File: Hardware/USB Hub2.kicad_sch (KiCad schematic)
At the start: 67 parts, among them J1 Conn_01x07_Male, J10 Conn_01x04_Male, J11 USB_C_Receptacle, J12 USB_C_Receptacle, J2 Conn_01x04_Male, J3 Conn_01x02_Male, J4 Conn_01x02_Male, J5 Conn_01x02_Male, J6 Conn_01x02_Male, J7 Conn_01x08_Male, J8 QWIIC_Vertical, J9 QWIIC_Stack_II, U1 TUSB2036, U2 AP2112K-3.3, U3 TPS2550DBVTG4, U4 TPS2550DBVTG4, U5 TPS2550DBVTG4, X1 ASE-48.000MHz

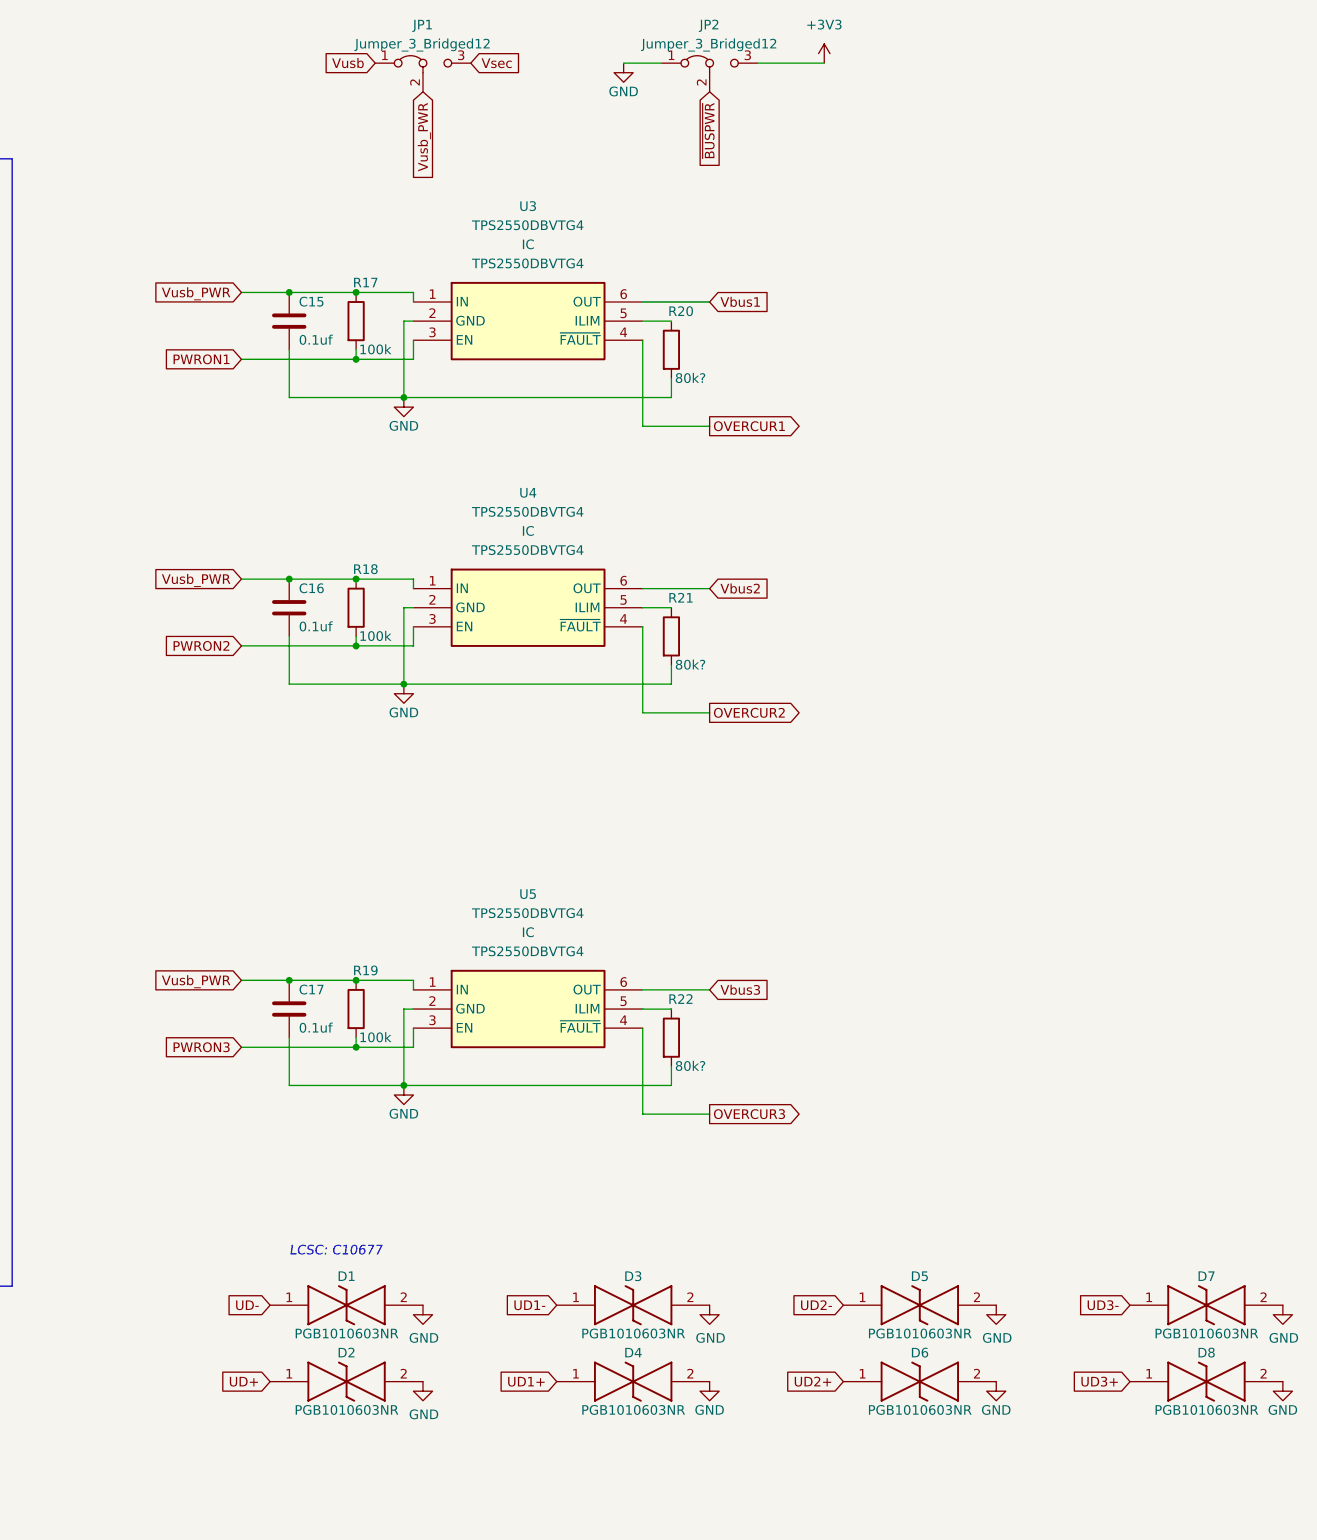
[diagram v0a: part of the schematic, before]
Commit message: Yay fer Hub2!
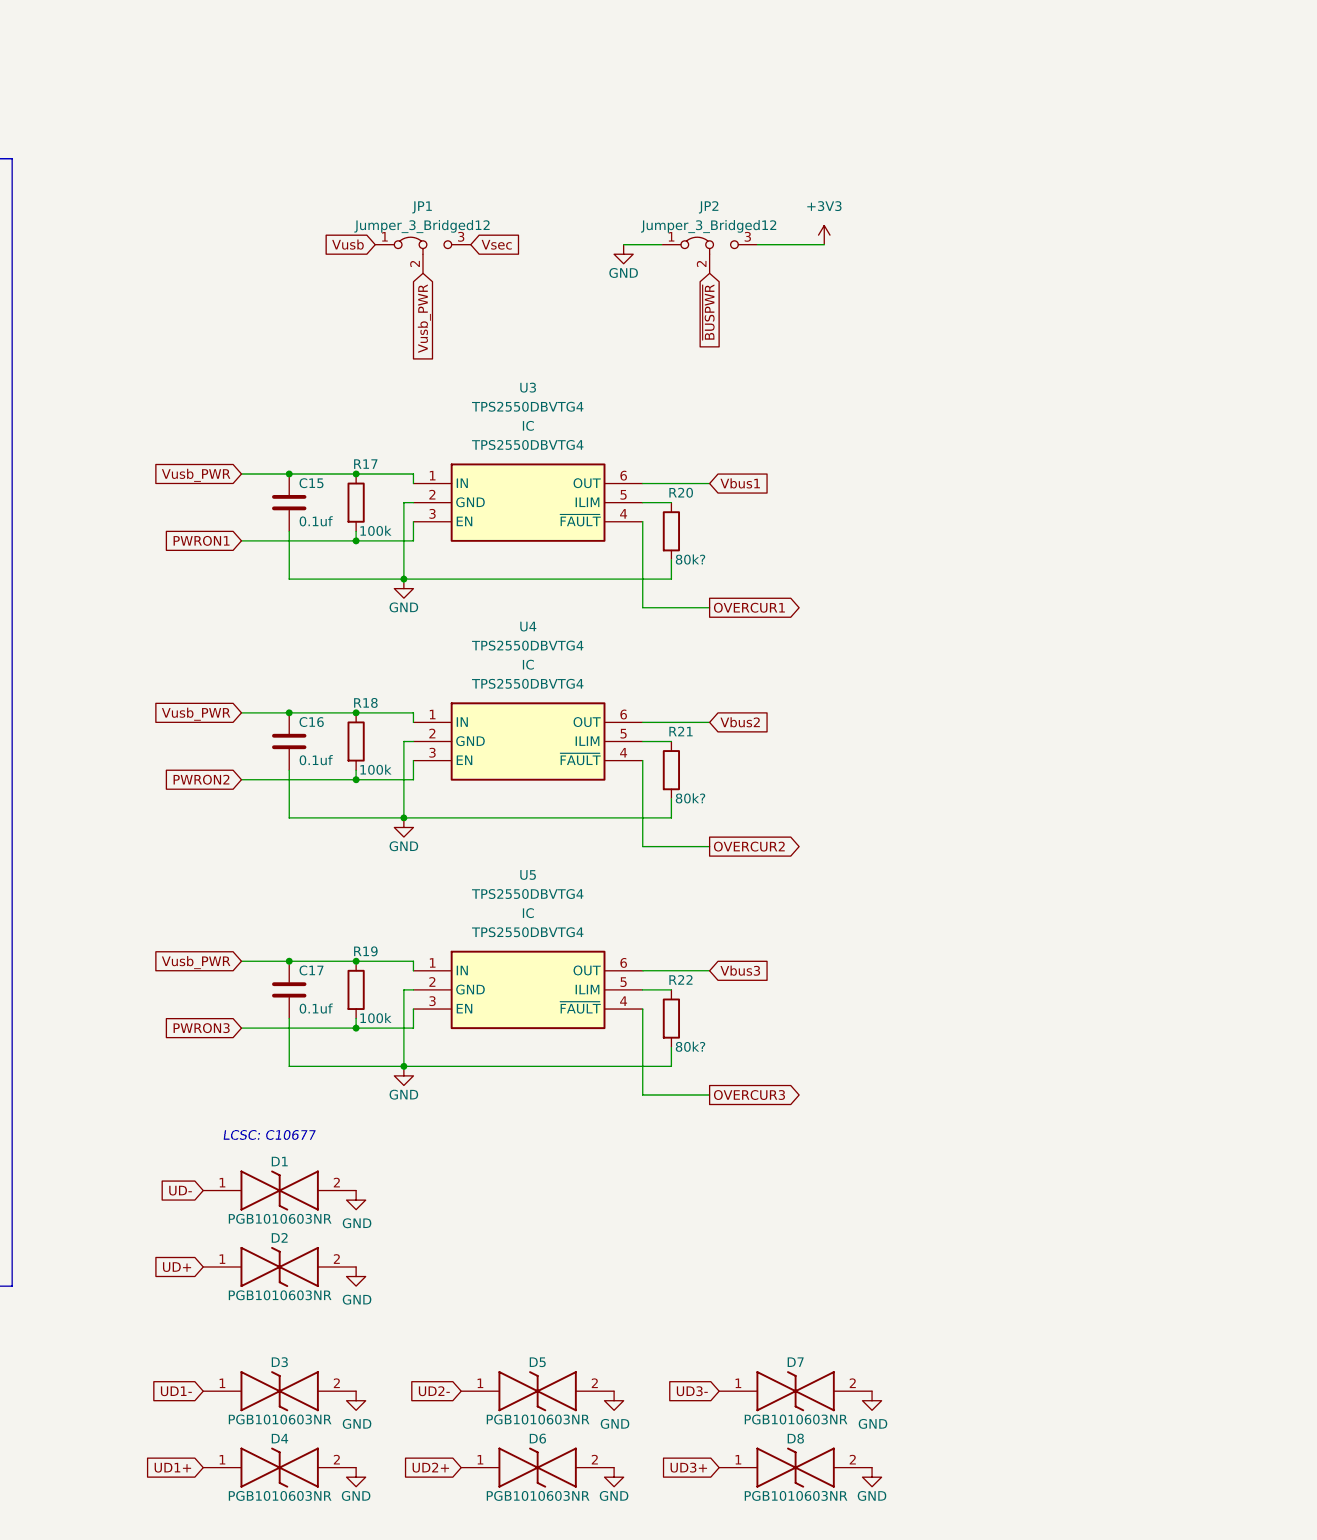
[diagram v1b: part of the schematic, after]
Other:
- moved on the sheet: C15, C16, C17, D1, D2, D3, D4, D5, D6, D7, D8, JP1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
